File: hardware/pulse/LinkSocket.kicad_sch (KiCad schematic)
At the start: 4 parts, among them J2001 2x05_Horizontal, U2001 THVD24x2

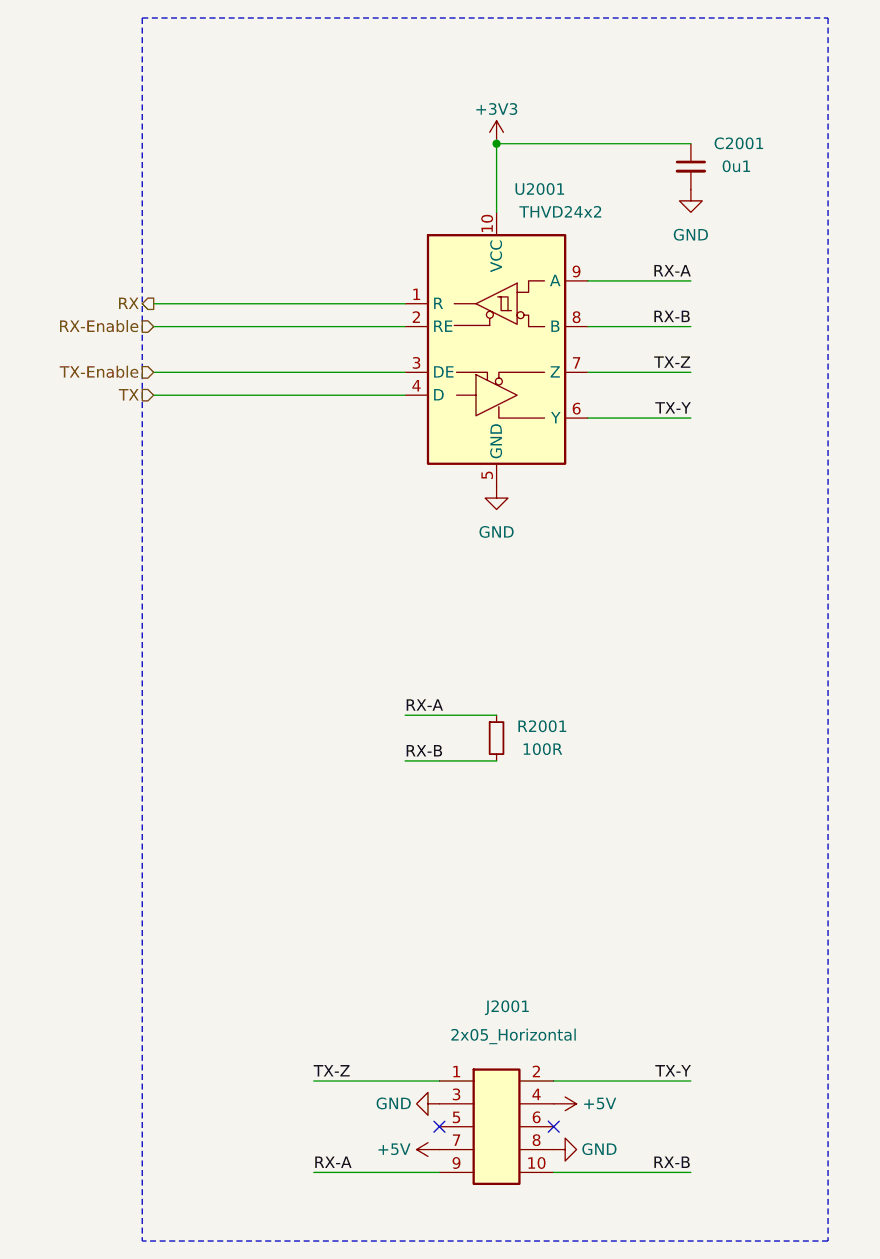
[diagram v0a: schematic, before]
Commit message: Update
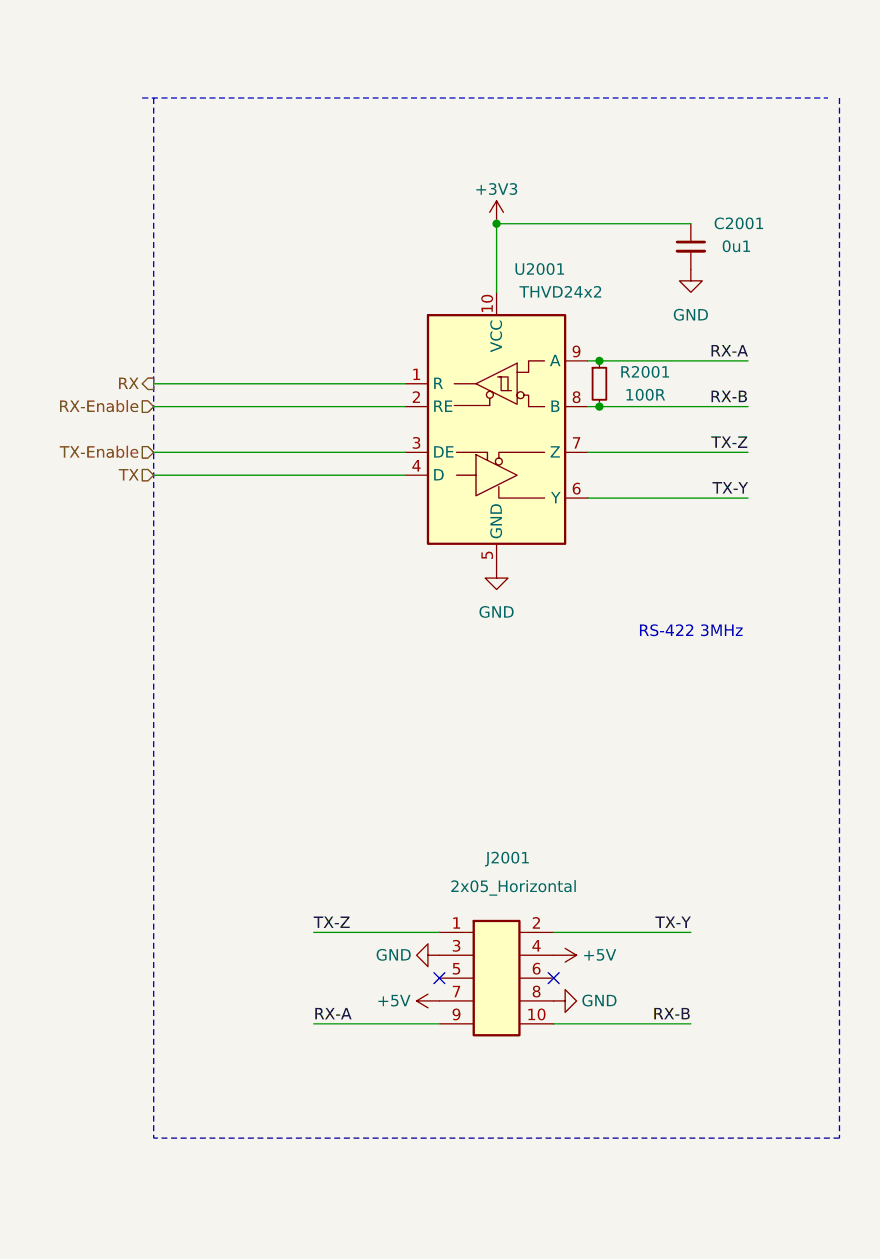
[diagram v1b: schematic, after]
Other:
- note added: "RS-422 3MHz"
- moved on the sheet: C2001, J2001, R2001, U2001

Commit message: Update parts
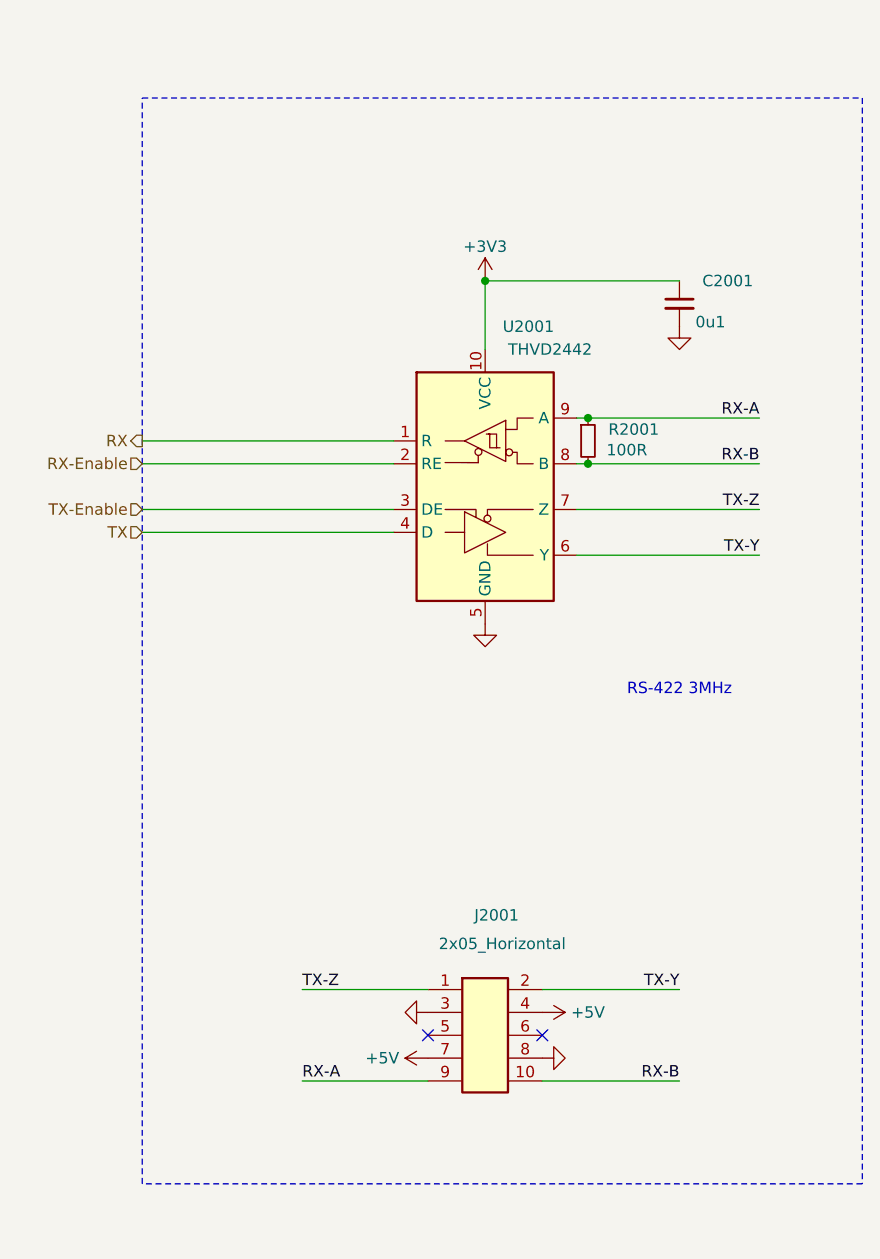
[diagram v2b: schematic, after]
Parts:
- C2001: footprint Capacitor_SMD:C_0603_1608Metric -> V2_Capacitor_SMD:C_0603; symbol Device:C_Small -> V2_Device:C_0603_0u1; Manufacturer (none) -> TDK; Mouser (none) -> 810-CGA3E2X7R1H104MA; Product (none) -> CGA3E2X7R1H104M080AA
- J2001: Manufacturer (none) -> Amphenol FCI; Mouser (none) -> 649-200211120001T4LF; Product (none) -> 20021112-00010T4LF
- R2001: footprint Resistor_SMD:R_0603_1608Metric -> V2_Resistor_SMD:R_0603; symbol Device:R_Small -> V2_Device:R_0603_100R; Manufacturer (none) -> Vishay; Mouser (none) -> 71-CRCW0603100RFKEAH; Product (none) -> CRCW0603100RFKEAHP; Rating (none) -> 330mW
- U2001: value THVD24x2 -> THVD2442; symbol V2_Interface_RS485:THVD24x2 -> V2_Interface_RS485:THVD2442; Manufacturer (none) -> Texas Instruments; Mouser (none) -> 595-THVD2442DRCR; Product (none) -> THVD2442DRCR
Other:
- moved on the sheet: C2001, J2001, R2001, U2001

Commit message: Update library
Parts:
- C2001: Rating (none) -> 50V
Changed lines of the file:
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@@
 			)
 		)
-		(property "Description" "Power symbol creates a global label with name \"+3V3\""
+		(property "Description" ""
 			(at 151.13 64.77 0)
 			(effects
@@
 			)
 		)
-		(property "Description" "Power symbol creates a global label with name \"GND\" , ground"
+		(property "Description" ""
 			(at 144.78 146.05 0)
 			(effects
@@
 			)
 		)
-		(property "Description" "Power symbol creates a global label with name \"GND\" , ground"
+		(property "Description" ""
 			(at 151.13 102.87 0)
 			(effects
@@
 			)
 		)
-		(property "Description" "Power symbol creates a global label with name \"GND\" , ground"
+		(property "Description" ""
 			(at 172.72 69.85 0)
 			(effects
@@
 			)
 		)
-		(property "Description" "Power symbol creates a global label with name \"GND\" , ground"
+		(property "Description" ""
 			(at 157.48 151.13 0)
 			(effects
@@
 			)
 		)
+		(property "Rating" "50V"
+			(at 172.72 90.17 0)
+			(effects
+				(font
+					(size 1.27 1.27)
+				)
+				(hide yes)
+			)
+		)
 		(pin "1"
 		)
@@
 			)
 		)
-		(property "Description" "Power symbol creates a global label with name \"+5V\""
+		(property "Description" ""
 			(at 144.78 151.13 0)
 			(effects
@@
 			)
 		)
-		(property "Description" "Power symbol creates a global label with name \"+5V\""
+		(property "Description" ""
 			(at 157.48 146.05 0)
 			(effects

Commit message: Update Library
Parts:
- C2001: symbol V2_Device:C_0603_0u1 -> V2_Capacitor:0603_0u1
- R2001: symbol V2_Device:R_0603_100R -> V2_Resistor:0603_100R
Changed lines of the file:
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@@
 	)
 	(symbol
-		(lib_id "V2_Device:R_0603_100R")
+		(lib_id "V2_Resistor:0603_100R")
 		(at 162.56 82.55 0)
 		(unit 1)
@@
 	)
 	(symbol
-		(lib_id "V2_Device:C_0603_0u1")
+		(lib_id "V2_Capacitor:0603_0u1")
 		(at 172.72 67.31 0)
 		(unit 1)

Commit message: Replace diode
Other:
- title: V2 Link -> V2 pulse
